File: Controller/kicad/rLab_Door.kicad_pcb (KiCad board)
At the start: 4 copper layers, 100 x 100 mm, 100 parts, among them J1 ACT_1, J10 BATTERY, J11 PROG, J12 PI, J13 TEST POINTS, J2 ACT_2, J3 NPX_1, J4 NPX_2, J5 WIEGAND KEYPAD, J6 NFC SERIAL, J7 I2C DISPLAY, J8 TAMPER, J9 V_IN, Q1 2N7002, Q10 MMBT5551L, Q11 2N7002, Q12 2N7002, Q2 2N7002, Q3 AO3401A, Q4 MMBT5551L, Q5 2N7002, Q6 2N7002, Q7 AO3401A, Q8 2N7002, Q9 2N7002, SW1 RESET, SW2 BOOT, SW3 TEST_1, SW4 TEST_2, U1 MP1584, U2 LM317_TO-252, U3 AMS1117-3.3, U4 ESP32-WROOM-32D

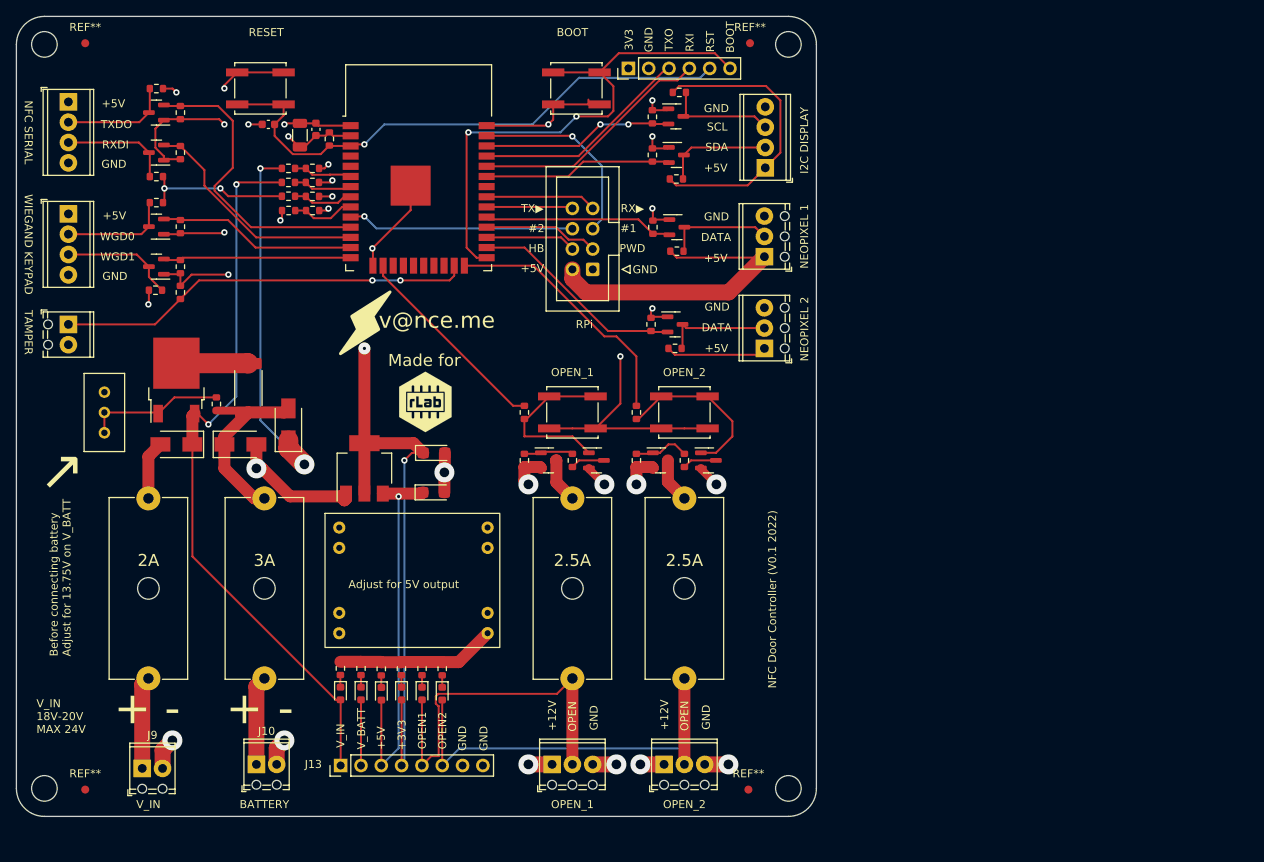
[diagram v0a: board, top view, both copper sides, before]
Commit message: Pre-production check-in
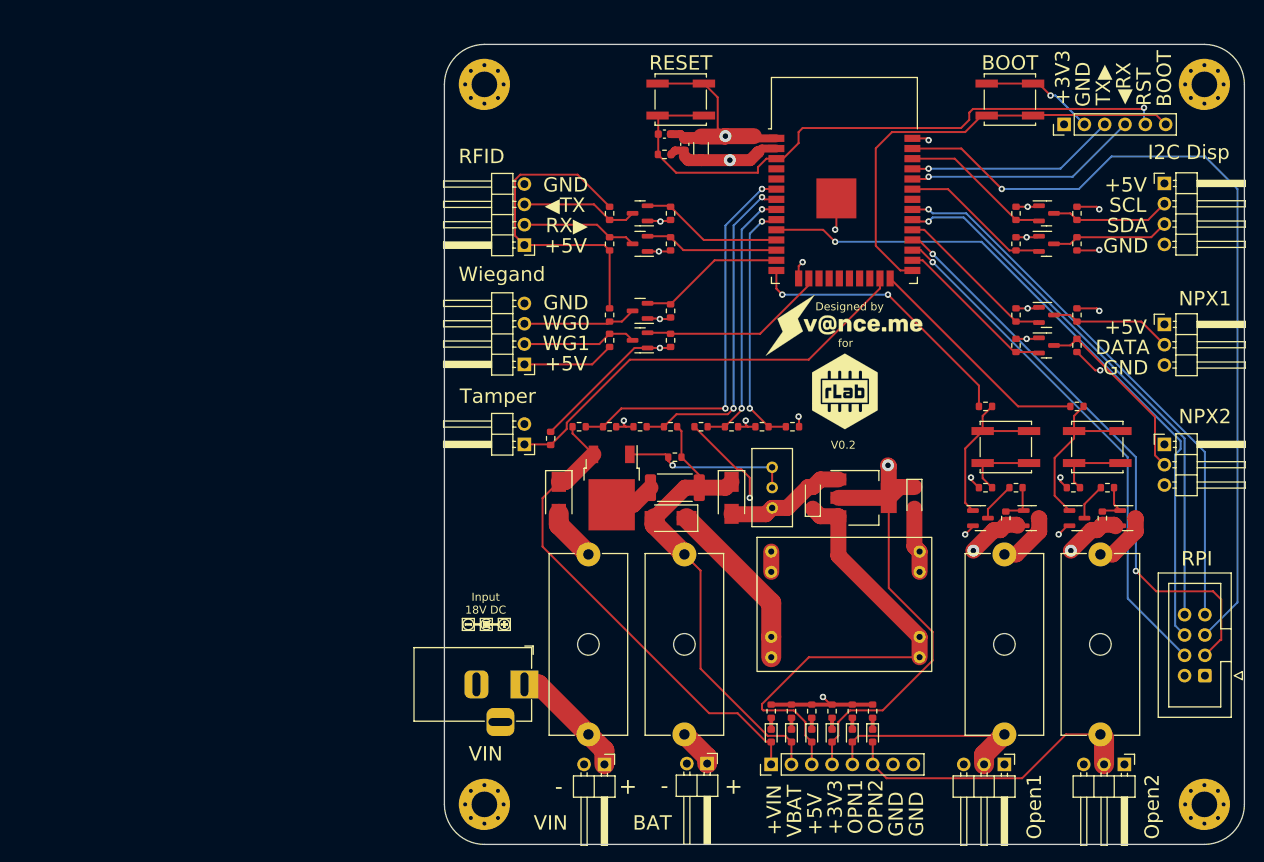
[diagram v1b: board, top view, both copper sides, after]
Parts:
- removed the REF** at (143.0, 50.0)
- removed the REF** at (50.0, 50.0)
- removed the REF** at (55.1, 143.2)
- removed the REF** at (50.0, 143.0)
- removed the REF** at (138.0, 143.2)
- removed the REF** at (55.1, 49.9)
- removed the REF** at (143.0, 143.0)
- removed the REF** at (138.2, 49.9)
- added J14: Jack-DC, Connector_BarrelJack:BarrelJack_Horizontal, F.Cu at (110.0, 130.0)
- added R41: 10k, Resistor_SMD:R_0603_1608Metric, F.Cu at (167.6, 105.4)
- added R42: 10k, Resistor_SMD:R_0603_1608Metric, F.Cu at (178.6, 105.4)
- added REF**: MountingHole_3.2mm_M3_Pad_Via, MountingHole:MountingHole_3.2mm_M3_Pad_Via, F.Cu at (195.0, 55.0)
- added REF**: MountingHole_3.2mm_M3_Pad_Via, MountingHole:MountingHole_3.2mm_M3_Pad_Via, F.Cu at (105.0, 55.0)
- added REF**: MountingHole_3.2mm_M3_Pad_Via, MountingHole:MountingHole_3.2mm_M3_Pad_Via, F.Cu at (195.0, 145.0)
- added REF**: MountingHole_3.2mm_M3_Pad_Via, MountingHole:MountingHole_3.2mm_M3_Pad_Via, F.Cu at (105.0, 145.0)
- J1, J2, J3, J4: footprint TerminalBlock_Phoenix:TerminalBlock_Phoenix_MPT-0,5-3-2.54_1x03_P2.54mm_Horizontal -> Connector_PinHeader_2.54mm:PinHeader_1x03_P2.54mm_Horizontal
- J10, J8, J9: footprint TerminalBlock_Phoenix:TerminalBlock_Phoenix_MPT-0,5-2-2.54_1x02_P2.54mm_Horizontal -> Connector_PinHeader_2.54mm:PinHeader_1x02_P2.54mm_Horizontal
- J5, J6, J7: footprint TerminalBlock_Phoenix:TerminalBlock_Phoenix_MPT-0,5-4-2.54_1x04_P2.54mm_Horizontal -> Connector_PinHeader_2.54mm:PinHeader_1x04_P2.54mm_Horizontal
- moved J12 91.8 mm to (195.1, 128.9)
- moved RV1 83.6 mm to (141.0, 102.9), turned to 90 degrees
- moved R14 68.5 mm to (143.5, 97.8), turned to 0 degrees
- moved R31 62.6 mm to (128.3, 71.1)
- moved U3 62.5 mm to (152.4, 106.7), turned to 0 degrees
- moved R17 62.3 mm to (139.7, 97.8)
- moved R33 62.3 mm to (128.3, 74.9)
- moved R26 62.2 mm to (128.3, 83.3)
- moved R28 62.0 mm to (128.3, 87.0)
- moved Q8 61.8 mm to (124.5, 71.1)
- moved D3 61.8 mm to (135.9, 106.7), turned to -90 degrees
- moved Q9 61.5 mm to (124.5, 74.9)
- moved Q5 61.4 mm to (124.5, 83.3)
- moved Q6 61.2 mm to (124.5, 87.0)
- moved Q3 60.8 mm to (173.4, 109.2)
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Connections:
- D2 pad 1: +BATT -> +12V
- D2 pad 2: Net-(D2-Pad2) -> V_BATT
- D3 pad 1: Net-(D2-Pad2) -> V_BATT
- D5 pad 2: +BATT -> V_BATT
- F2 pad 1: Net-(D2-Pad2) -> V_BATT
- J1 pad 1: +BATT -> +12V
- J13 pad 2: +BATT -> V_BATT
- J2 pad 1: +BATT -> +12V
- J5 pad 2: WG_D0_5 -> WG_D1_5
- J5 pad 3: WG_D1_5 -> WG_D0_5
- J6 pad 2: TXDO_NFC_5 -> RXDI_NFC_5
- J6 pad 3: RXDI_NFC_5 -> TXDO_NFC_5
- J7 pad 2: SDA_DISP_5 -> SCL_DISP_5
- J7 pad 3: SCL_DISP_5 -> SDA_DISP_5
- Q3 pad 2: +BATT -> +12V
- Q7 pad 2: +BATT -> +12V
- R17 pad 1: GND -> ADC_V3
- R17 pad 2: ADC_V3 -> GND
- R19 pad 1: +BATT -> +12V
- R2 pad 2: Net-(D2-Pad2) -> V_BATT
- R3 pad 1: Net-(D2-Pad2) -> V_BATT
- R30 pad 1: +BATT -> +12V
- R6 pad 2: +BATT -> V_BATT
- SW3 pad 2: +3V3 -> Net-(R41-Pad1)
- SW4 pad 2: +3V3 -> Net-(R42-Pad1)
- U1 pad 1: +BATT -> +12V
- U4 pad 14: WG_D1 -> OPEN_1
- U4 pad 16: OPEN_1 -> WG_D1
- U4 pad 6: ADC_VBATT -> ADC_VIN
- U4 pad 7: ADC_VIN -> ADC_VBATT
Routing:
- net PI_OPEN_CMD_1: track 24.3 -> 103.5 mm
- net +BATT: track 68.7 -> 0.00 mm, vias 6 -> 0
- net V_BATT: track 0.00 -> 59.4 mm
- net PI_POWERED: track 14.4 -> 73.5 mm, vias 0 -> 2
- net PI_OPEN_CMD_2: track 28.4 -> 86.5 mm
- net TXDO_PI: track 10.8 -> 67.8 mm, vias 0 -> 1
- net RXDI_PI: track 13.8 -> 69.5 mm, vias 0 -> 1
- net PI_HEARTBEAT: track 11.3 -> 65.3 mm, vias 0 -> 1
- net +3V3: track 163.6 -> 116.2 mm, vias 12 -> 13
- net ADC_VIN: track 7.40 -> 49.5 mm, vias 0 -> 2
- net +12V: track 0.00 -> 38.0 mm, vias 0 -> 2
- net ADC_VBATT: track 7.38 -> 41.6 mm, vias 0 -> 2
- net V_IN: track 91.6 -> 60.2 mm, vias 2 -> 0
- net +5V: track 164.8 -> 136.6 mm
- net ADC_V5: track 7.60 -> 33.1 mm, vias 0 -> 2
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- added copper zone on In2.Cu, net +12V
- added copper zone on In2.Cu, net GND
- removed copper zone on In2.Cu, net +BATT
- removed copper zone on In2.Cu, net Net-(F1-Pad2)
- removed copper zone on In2.Cu, net Net-(F2-Pad2)
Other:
- outline, holes or cut-outs redrawn
- board text added: "+VIN"
- board text added: "BAT"
- board text added: "Battery"
- board text added: "Designed by"
- board text added: "I2C Disp"
- board text added: "Input 18V DC"
- board text added: "NPX1"
- board text added: "NPX2"
- board text added: "Neopix1"
- board text added: "Neopix2"
- board text added: "OPN1"
- board text added: "OPN2"
- board text added: "Open1"
- board text added: "Open2"
- board text added: "Program"
- board text added: "RFID"
- board text added: "RPI"
- board text added: "Rasp Pi"
- board text added: "SW#1"
- board text added: "SW#2"
- board text added: "Tamper"
- board text added: "Testpoints"
- board text added: "V0.2"
- board text added: "VBAT"
- board text added: "VIN"
- board text added: "VIN supplied through barrel jack or 0.1"
- board text added: "WG0"
- board text added: "WG1"
- board text added: "Wiegand"
- board text added: "for"
- board text added: "◀RX"
- board text added: "◀TX"
- board text removed: "#1"
- board text removed: "#2"
- board text removed: "2.5A"
- board text removed: "2A"
- board text removed: "3A"
- board text removed: "3V3"
- board text removed: "Adjust for 5V output"
- board text removed: "BATTERY"
- board text removed: "Before connecting battery Adjust for 13.75V on V_BATT"
- board text removed: "HB"
- board text removed: "I2C DISPLAY"
- board text removed: "Made for"
- board text removed: "NEOPIXEL 1"
- board text removed: "NEOPIXEL 2"
- board text removed: "NFC Door Controller (V0.1 2022)"
- board text removed: "NFC SERIAL"
- board text removed: "OPEN"
- board text removed: "OPEN1"
- board text removed: "OPEN2"
- board text removed: "OPEN_1"
- board text removed: "OPEN_2"
- board text removed: "PWD"
- board text removed: "RPi"
- board text removed: "RXDI"
- board text removed: "RXI"
- board text removed: "TAMPER"
- board text removed: "TXDO"
- board text removed: "TXO"
- board text removed: "V_BATT"
- board text removed: "V_IN"
- board text removed: "V_IN 18V-20V MAX 24V"
- board text removed: "WGD0"
- board text removed: "WGD1"
- board text removed: "WIEGAND KEYPAD"
- board text removed: "v@nce.me"
- board text removed: "↘"
